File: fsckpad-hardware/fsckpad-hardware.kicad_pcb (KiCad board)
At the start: 2 copper layers, 158.1 x 78.3 mm, 55 parts, among them IC1 LS20-S, IC3 ICM-42670-P, IC4 PCA9555D, IC5 PCA9555D, IC6 LS20-S, U1 DRV2605LDGS, X1 1-TS009, Y1 1-TS009

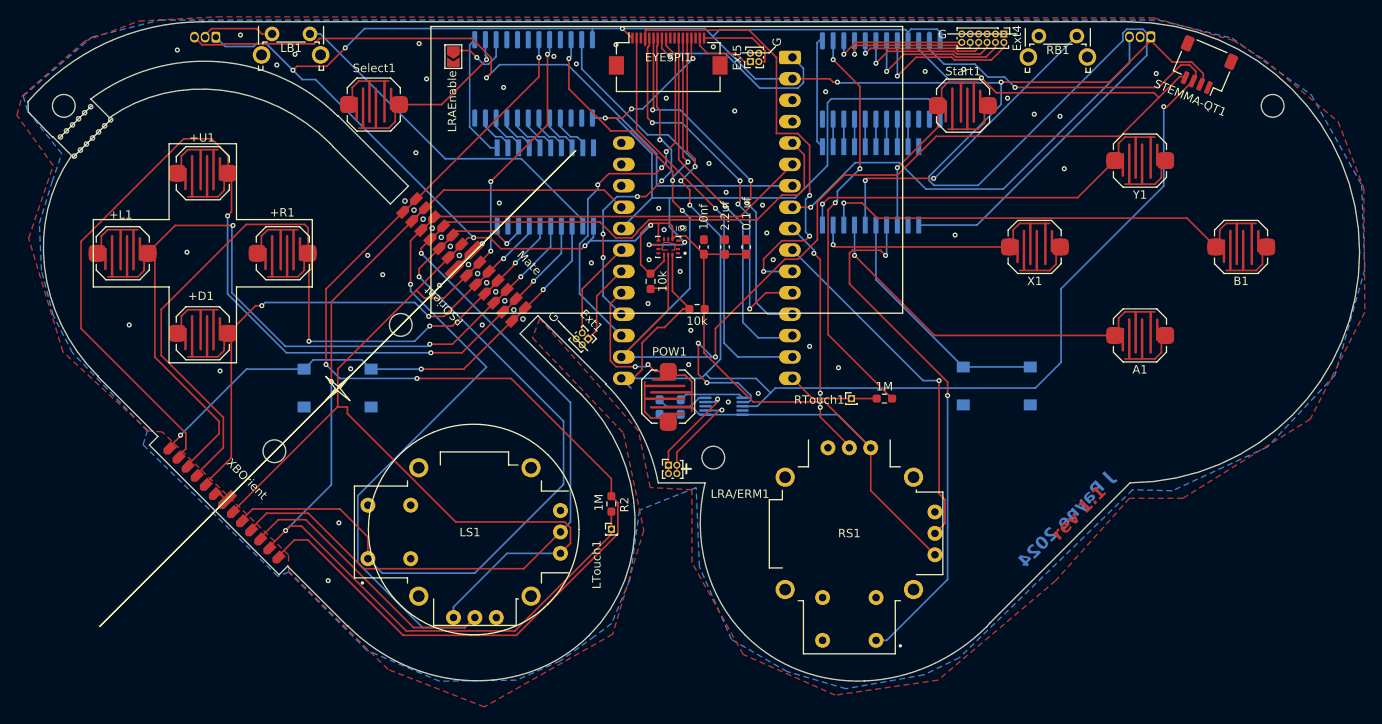
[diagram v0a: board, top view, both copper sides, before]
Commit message: rev 1
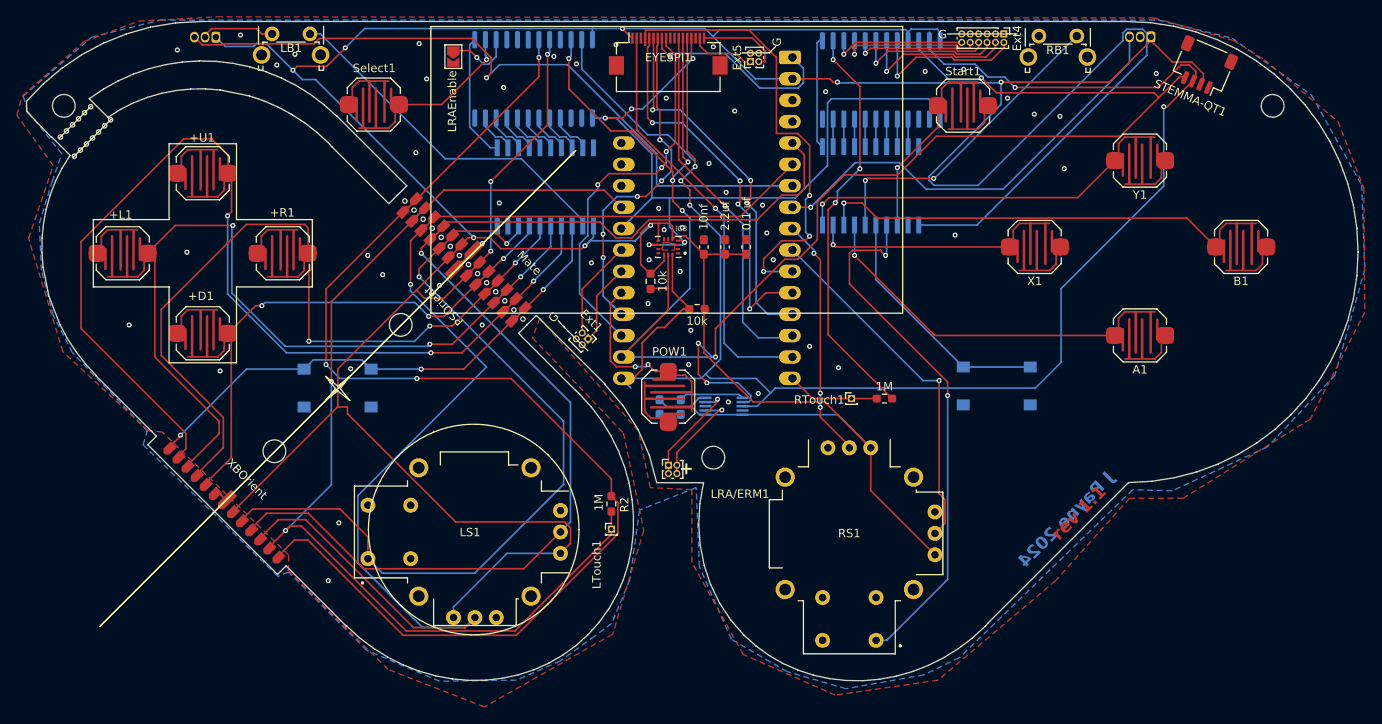
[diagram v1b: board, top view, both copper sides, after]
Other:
- outline, holes or cut-outs redrawn
